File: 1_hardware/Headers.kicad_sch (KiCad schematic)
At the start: 18 parts, among them J111 SSW-132-24-L-D, J121 SSW-132-24-L-D, J2 Power, J3 Buttons, J4 Reserve1, J5 Reserve2

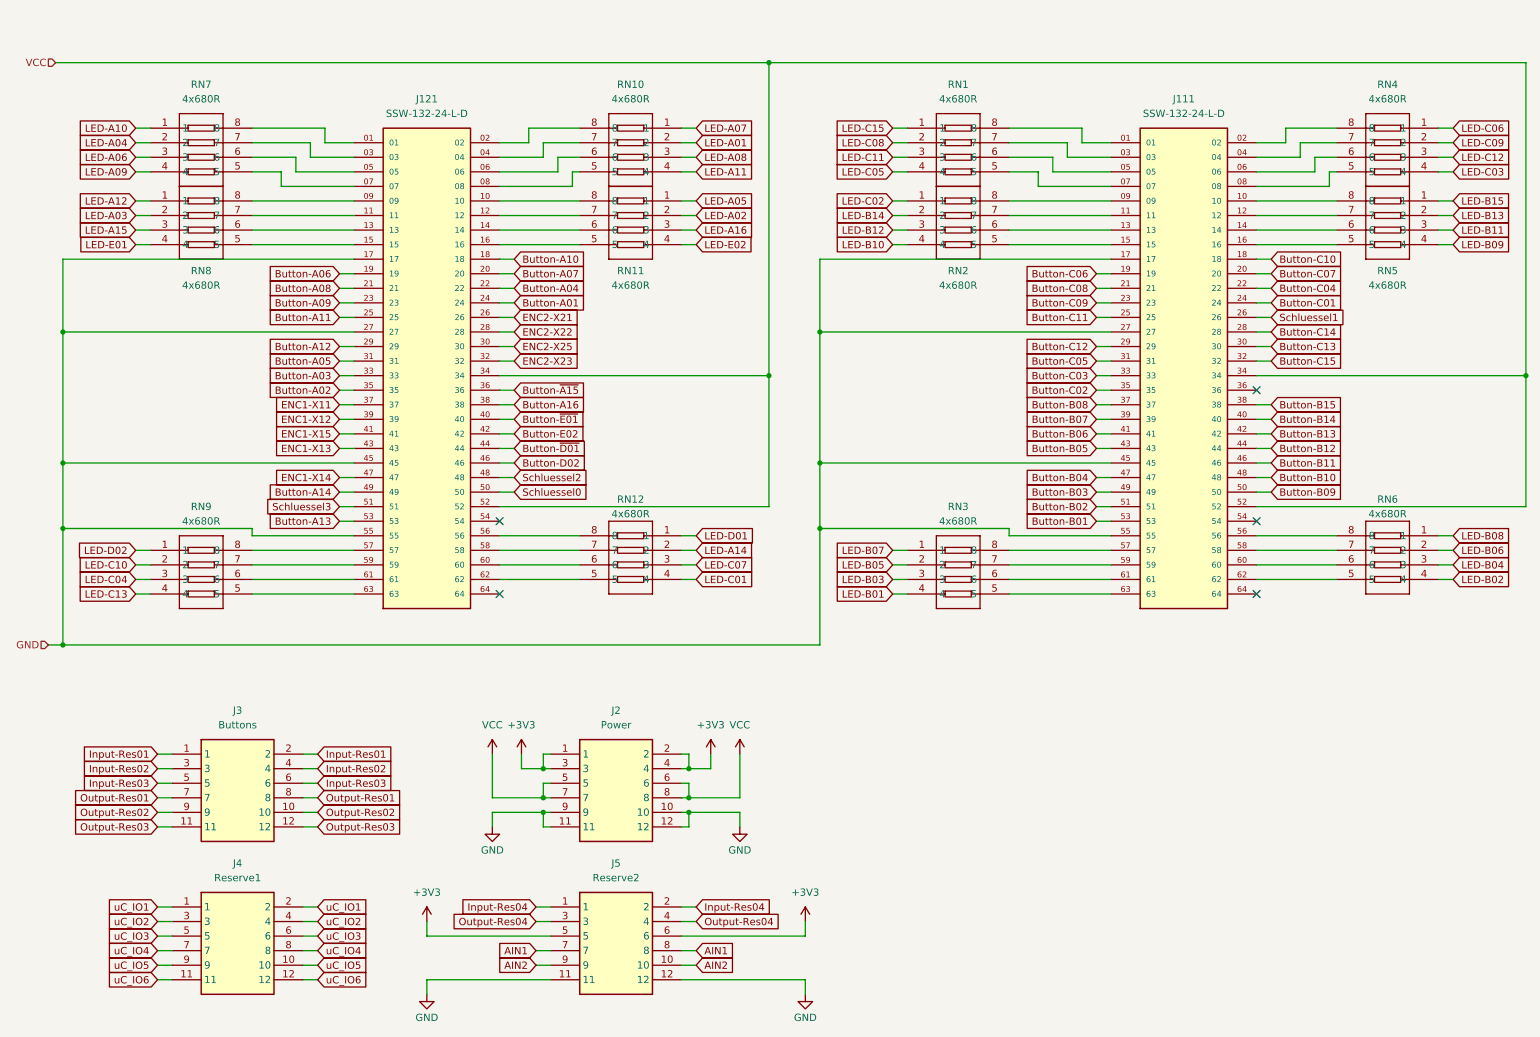
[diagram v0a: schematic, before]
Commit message: finished schematics and board
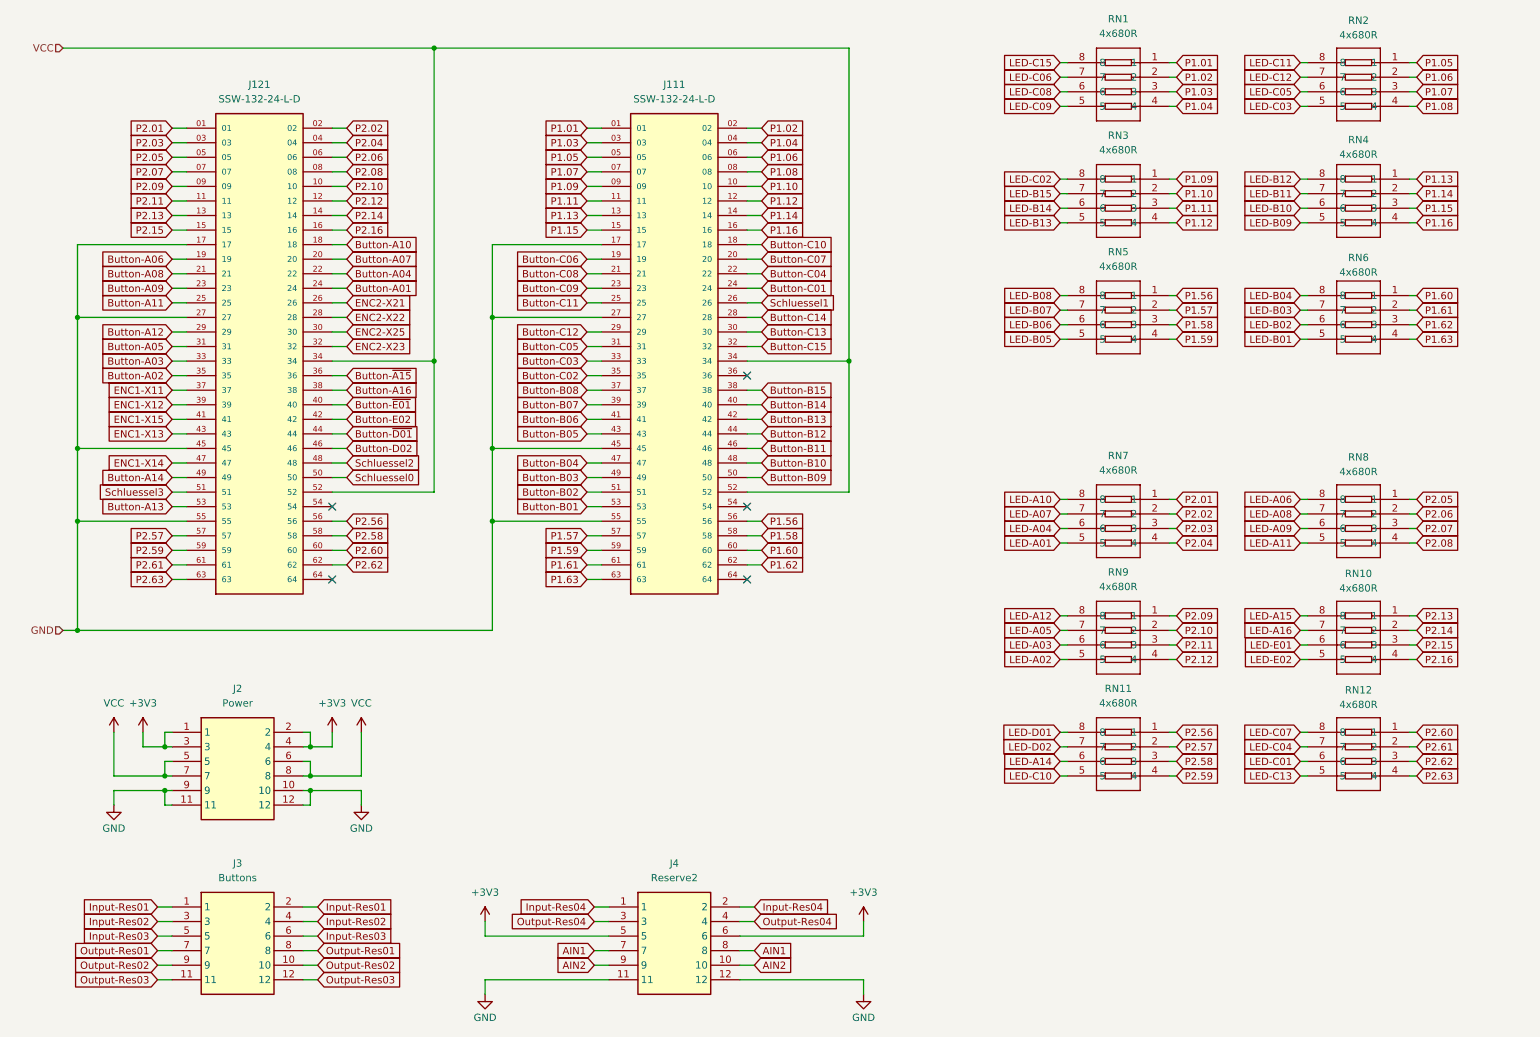
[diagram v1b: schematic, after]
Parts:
- removed J4: Reserve1, CostumLibrary:1824460000 - LSF-SMT 3.500690 3.5SN BK TU, symbol CostumLibrary:1824460000 - LSF-SMT 3.50/06/90 3.5SN BK TU
- renumbered J5 to J4
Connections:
- net LED-A01: now also RN7.5; no longer RN10.2
- net LED-A02: now also RN9.5; no longer RN11.2
- net LED-A03: now also RN9.6; no longer RN8.2
- net LED-A04: now also RN7.6; no longer RN7.2
- net LED-A05: now also RN9.7; no longer RN11.1
- net LED-A06: now also RN8.8; no longer RN7.3
- net LED-A07: now also RN7.7; no longer RN10.1
- net LED-A08: now also RN8.7; no longer RN10.3
- net LED-A09: now also RN8.6; no longer RN7.4
- net LED-A10: now also RN7.8; no longer RN7.1
- net LED-A11: now also RN8.5; no longer RN10.4
- net LED-A12: now also RN9.8; no longer RN8.1
- net LED-A14: now also RN11.6; no longer RN12.2
- net LED-A15: now also RN10.8; no longer RN8.3
- net LED-A16: now also RN10.7; no longer RN11.3
- net LED-B01: now also RN6.5; no longer RN3.4
- net LED-B02: now also RN6.6; no longer RN6.4
- net LED-B03: now also RN6.7; no longer RN3.3
- net LED-B04: now also RN6.8; no longer RN6.3
- net LED-B05: now also RN5.5; no longer RN3.2
- net LED-B06: now also RN5.6; no longer RN6.2
- net LED-B07: now also RN5.7; no longer RN3.1
- net LED-B08: now also RN5.8; no longer RN6.1
- net LED-B09: now also RN4.5; no longer RN5.4
- net LED-B10: now also RN4.6; no longer RN2.4
- net LED-B11: now also RN4.7; no longer RN5.3
- net LED-B12: now also RN4.8; no longer RN2.3
- net LED-B13: now also RN3.5; no longer RN5.2
- net LED-B14: now also RN3.6; no longer RN2.2
- net LED-B15: now also RN3.7; no longer RN5.1
- net LED-C01: now also RN12.6; no longer RN12.4
- net LED-C02: now also RN3.8; no longer RN2.1
- net LED-C03: now also RN2.5; no longer RN4.4
- net LED-C04: now also RN12.7; no longer RN9.3
- net LED-C05: now also RN2.6; no longer RN1.4
- net LED-C06: now also RN1.7; no longer RN4.1
- net LED-C07: now also RN12.8; no longer RN12.3
- net LED-C08: now also RN1.6; no longer RN1.2
- net LED-C09: now also RN1.5; no longer RN4.2
- net LED-C10: now also RN11.5; no longer RN9.2
- net LED-C11: now also RN2.8; no longer RN1.3
- net LED-C12: now also RN2.7; no longer RN4.3
- net LED-C13: now also RN12.5; no longer RN9.4
- net LED-C15: now also RN1.8; no longer RN1.1
- net LED-D01: now also RN11.8; no longer RN12.1
- net LED-D02: now also RN11.7; no longer RN9.1
- net LED-E01: now also RN10.6; no longer RN8.4
- net LED-E02: now also RN10.5; no longer RN11.4
- net P2.15: now reaches J121.15
- net P2.15: now also RN10.3; no longer RN8.5
- net P2.13: now reaches J121.13
- net P2.13: now also RN10.1; no longer RN8.6
- net P2.11: now reaches J121.11
- net P2.11: now also RN9.3; no longer RN8.7
- net P2.09: now reaches J121.09
- net P2.09: now also RN9.1; no longer RN8.8
- net P2.08: now reaches J121.08
- net P2.08: now also RN8.4; no longer RN10.5
- net P2.06: now reaches J121.06
- net P2.06: now also RN8.2; no longer RN10.6
- net P2.04: now reaches J121.04
- net P2.04: now also RN7.4; no longer RN10.7
- net P2.02: now reaches J121.02
- net P2.02: now also RN7.2; no longer RN10.8
- net P2.16: now reaches J121.16
- net P2.16: now also RN10.4; no longer RN11.5
- net P2.14: now reaches J121.14
- net P2.14: now also RN10.2; no longer RN11.6
- net P2.12: now reaches J121.12
- net P2.12: now also RN9.4; no longer RN11.7
- net P2.10: now reaches J121.10
- net P2.10: now also RN9.2; no longer RN11.8
- net P2.07: now reaches J121.07
- net P2.07: now also RN8.3; no longer RN7.5
- net P2.05: now reaches J121.05
- net P2.05: now also RN8.1; no longer RN7.6
- net P2.03: now reaches J121.03
- net P2.03: now also RN7.3; no longer RN7.7
- net P2.01: now reaches J121.01
- net P2.01: now also RN7.1; no longer RN7.8
- net P2.62: now reaches J121.62
- net P2.62: now also RN12.3; no longer RN12.5
- net P2.60: now reaches J121.60
- net P2.60: now also RN12.1; no longer RN12.6
- net P2.58: now reaches J121.58
- net P2.58: now also RN11.3; no longer RN12.7
- net P2.56: now reaches J121.56
- net P2.56: now also RN11.1; no longer RN12.8
- net P1.16: now reaches J111.16
- net P1.16: now also RN4.4; no longer RN5.5
- net P1.14: now reaches J111.14
- net P1.14: now also RN4.2; no longer RN5.6
- net P1.12: now reaches J111.12
- net P1.12: now also RN3.4; no longer RN5.7
- net P1.10: now reaches J111.10
- net P1.10: now also RN3.2; no longer RN5.8
- net P2.57: now reaches J121.57
- net P2.57: now also RN11.2; no longer RN9.8
- net P2.59: now reaches J121.59
- net P2.59: now also RN11.4; no longer RN9.7
- net P2.61: now reaches J121.61
- net P2.61: now also RN12.2; no longer RN9.6
- net P2.63: now reaches J121.63
- net P2.63: now also RN12.4; no longer RN9.5
- net P1.15: now reaches J111.15
- net P1.15: now also RN4.3; no longer RN2.5
- net P1.13: now reaches J111.13
- net P1.13: now also RN4.1; no longer RN2.6
- net P1.11: now reaches J111.11
- net P1.11: now also RN3.3; no longer RN2.7
- net P1.09: now reaches J111.09
- net P1.09: now also RN3.1; no longer RN2.8
- net P1.08: now reaches J111.08
- net P1.08: now also RN2.4; no longer RN4.5
- net P1.06: now reaches J111.06
- net P1.06: now also RN2.2; no longer RN4.6
- net P1.04: now reaches J111.04
- net P1.04: now also RN1.4; no longer RN4.7
- net P1.02: now reaches J111.02
- net P1.02: now also RN1.2; no longer RN4.8
- net P1.62: now reaches J111.62
- net P1.62: now also RN6.3; no longer RN6.5
- net P1.60: now reaches J111.60
- net P1.60: now also RN6.1; no longer RN6.6
- net P1.58: now reaches J111.58
- net P1.58: now also RN5.3; no longer RN6.7
- net P1.56: now reaches J111.56
- net P1.56: now also RN5.1; no longer RN6.8
- net P1.07: now reaches J111.07
- net P1.07: now also RN2.3; no longer RN1.5
- net P1.05: now reaches J111.05
- net P1.05: now also RN2.1; no longer RN1.6
- net P1.03: now reaches J111.03
- net P1.03: now also RN1.3; no longer RN1.7
- net P1.01: now reaches J111.01
- net P1.01: now also RN1.1; no longer RN1.8
- net P1.63: now reaches J111.63
- net P1.63: now also RN6.4; no longer RN3.5
- net P1.61: now reaches J111.61
- net P1.61: now also RN6.2; no longer RN3.6
- net P1.59: now reaches J111.59
- net P1.59: now also RN5.4; no longer RN3.7
- net P1.57: now reaches J111.57
- net P1.57: now also RN5.2; no longer RN3.8
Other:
- moved on the sheet: J111, J121, J2, J3, J4
